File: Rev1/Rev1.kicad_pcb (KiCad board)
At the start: 2 copper layers, 71.7 x 72.8 mm, 142 parts, among them CON1 NA(NH1x20), J1 Conn_02x02_P4.20mm_Molex_Hori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, Q1 Q12MHz/20pF/30ppm/2P/HC-49SM(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, Q2 BC817-40(SOT23), Q3 BC817-40(SOT23), T1 DTC114YKA, U1 USB-C-16P-F(A40-00119-A52-12), U2 K7805-2000R3L, U3 CH340T(SSOP20W), U4 LAN8710A-EZC(QFN32), U5 K7803-2000R3L, U6 TCA9548APWR, U7 ESP32-WROOM-32D-4MB

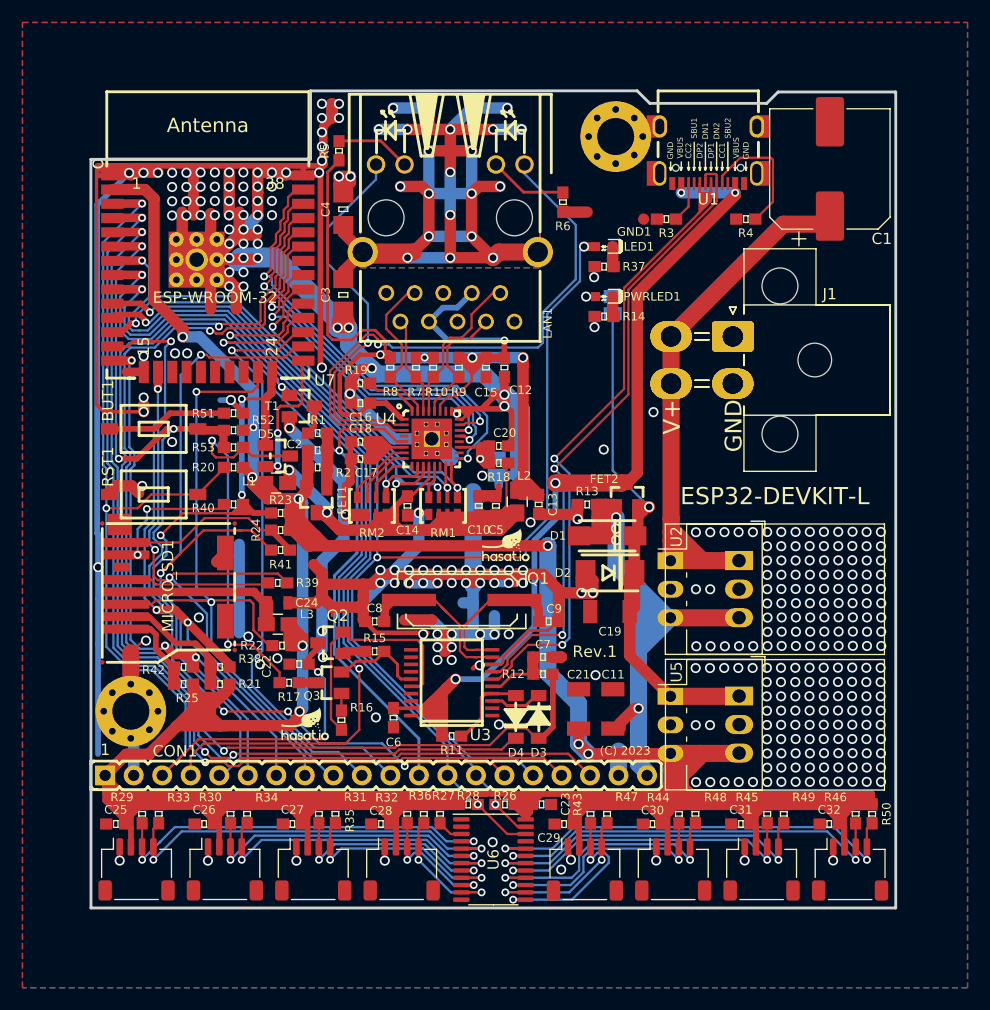
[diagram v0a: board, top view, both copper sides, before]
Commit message: .
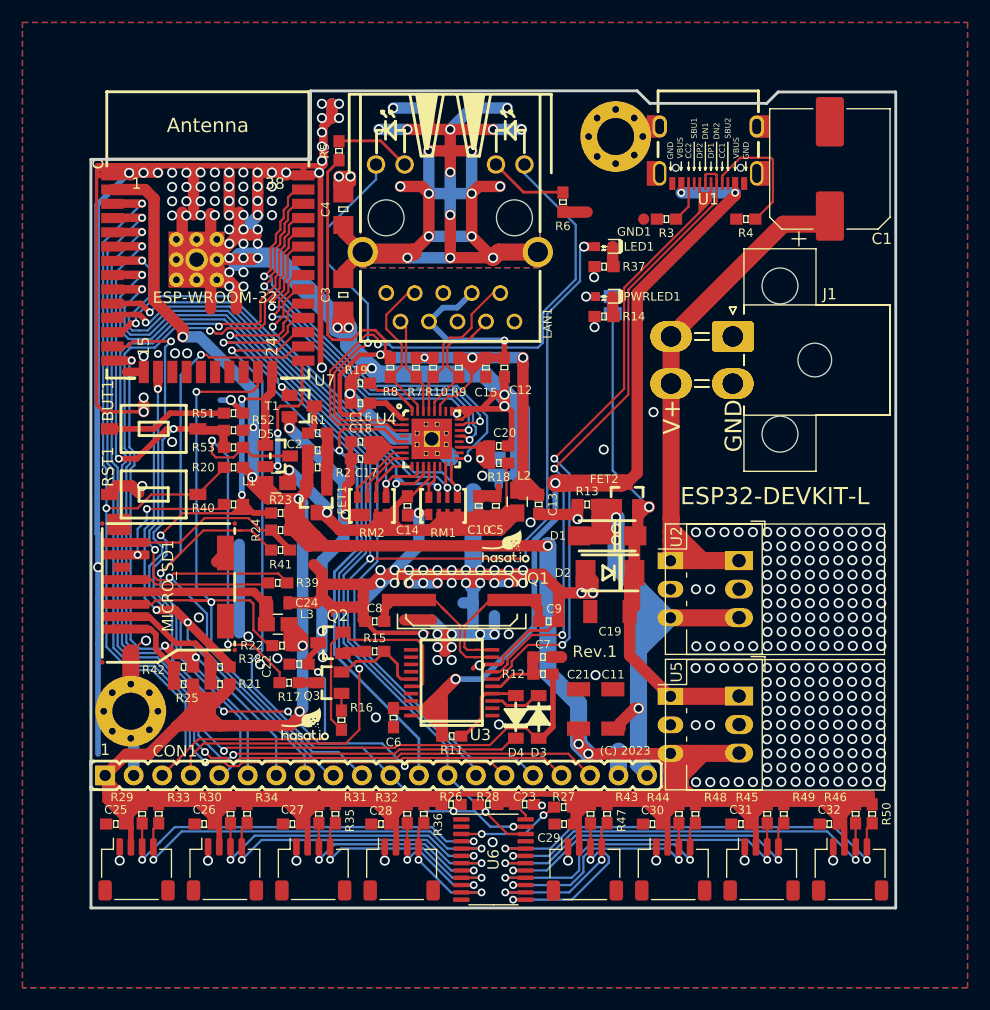
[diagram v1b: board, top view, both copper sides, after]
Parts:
- U2: value K7805-2000R3L -> Converter_DCDC_RECOM_R-78HB-0.5L_THT
- moved R27 11.0 mm to (111.7, 130.8), turned to 180 degrees
- moved R28 1.53 mm to (104.9, 130.6)
- moved R26 1.53 mm to (101.7, 130.6)
- moved C23 1.51 mm to (108.2, 130.6)
- moved G*** 0.11 mm to (106.6, 107.6)
- renumbered R28 to R26, R26 to R28
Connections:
- net /GPIO34\BUT1 renamed /GPI34\BUT1
- net /GPIO36 renamed /GPI36
- net /GPIO39 renamed /GPI39
- CON1 pad 14: /GPIO33 -> /GPIO33\LED
- CON1 pad 16: /GPIO35\LED -> /GPI35
- LED1 pad 2: /GPIO35\LED -> /GPIO33\LED
- R26 pad 2: /GPIO32 -> /GPIO16
- R28 pad 2: /GPIO33 -> /GPIO32
- U6 pad 23: /GPIO33 -> /GPIO16
- U7 pad 7: /GPIO35\LED -> /GPI35
- U7 pad 9: /GPIO33 -> /GPIO33\LED
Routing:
- net /GPIO35\LED: track 120.3 -> 0.00 mm, vias 4 -> 0
- net /GPIO33\LED: track 0.00 -> 113.5 mm, vias 0 -> 4
- net +3V3: track 721.5 -> 639.4 mm
- net /GPI35: track 0.00 -> 76.0 mm, vias 0 -> 1
- net /GPIO33: track 75.5 -> 0.00 mm, vias 2 -> 0
- net /GPIO16: track 54.1 -> 68.9 mm, vias 1 -> 3
- net Net-(U6-~{RESET}): track 2.29 -> 9.46 mm, vias 0 -> 2
- net /GPIO32: track 78.5 -> 79.4 mm
